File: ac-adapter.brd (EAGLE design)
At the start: 113 x 52.7 mm, 96 parts, among them IC1 UCC256404A, IC2 TL431, Q1 200V 3A, Q3 TLP621-1, T1 COMMON_FILTER-SU10VFC, T2 TRANSFORMAER_FLYBACK-ETD34

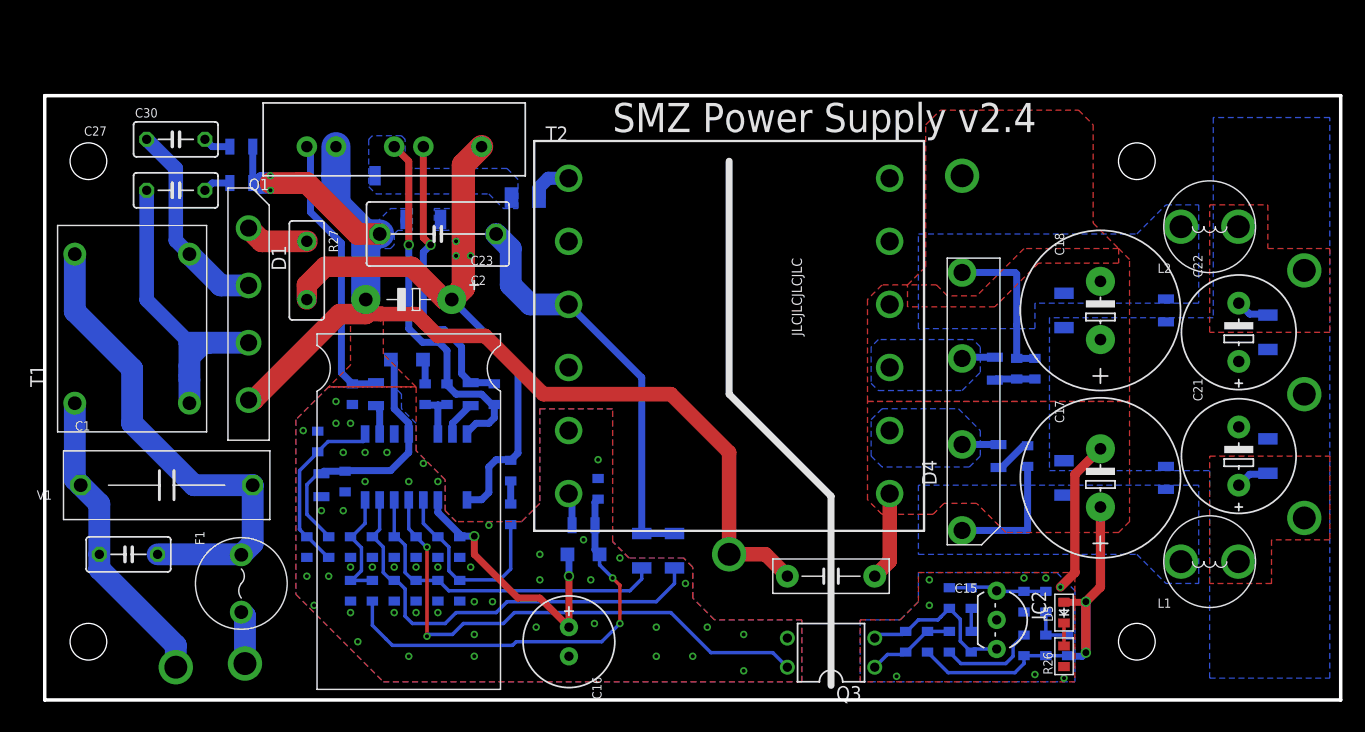
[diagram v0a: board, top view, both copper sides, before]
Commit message: 曲げた
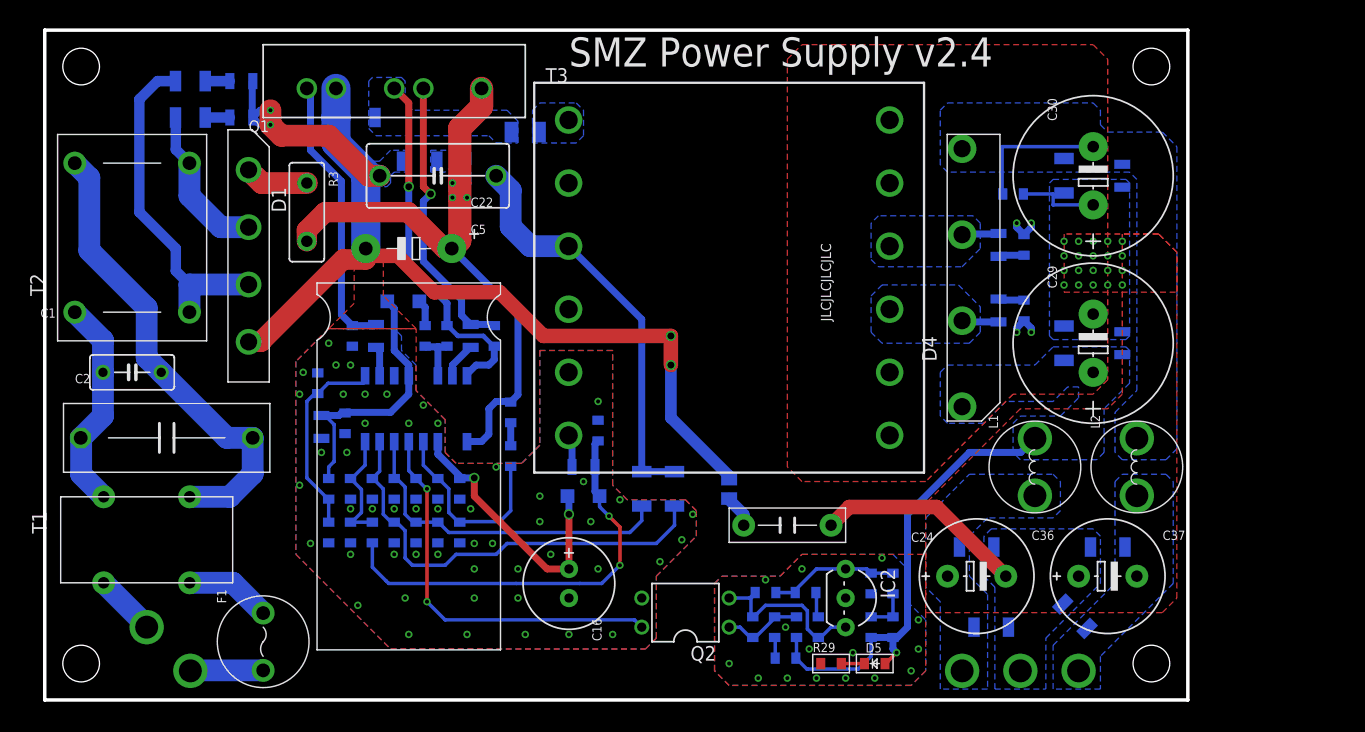
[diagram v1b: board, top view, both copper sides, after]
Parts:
- removed Q3: TLP621-1, my_ic:DIL04
- removed TP6: GND, my_connector:TESTPIN-LARGE
- removed TP7: PGND, my_connector:TESTPIN-LARGE
- removed V1: Varistor, my_rcl:C050
- added C40, C41, C42: 10u, my_rcl:3225-2
- added FB2: FB-3216, my_rcl:3216-J
- added Q2: TLP621-1, my_ic:DIL04
- added T3: TRANSFORMAER_FLYBACK-ETD34, my_rcl:BETD34LLC
- C1: value 0.22uX -> Varistor; device my_rcl:X-CAPACITER -> my_rcl:C050
- C10: value 10p -> 1u
- C11: value DNP -> 0.1u
- C12: value 22p -> 10u; device my_rcl:1608 -> my_rcl:2012
- C13: value 1kV 1000p -> 1u; device my_rcl:3225 -> my_rcl:1608
- C14: value 10p -> 1kV 1000p; device my_rcl:1608 -> my_rcl:3225
- C15: value 1000pY -> 1kV 1000p; device my_rcl:Y-CAPACITER -> my_rcl:3225
- C17: value 1000u -> 220p 1kV; device my_rcl:E5-13 -> my_rcl:3225
- C18: value 1000u -> 10p; device my_rcl:E5-13 -> my_rcl:1608
- C19: value 1000p -> 100p 1kV; device my_rcl:1608 -> my_rcl:3225
- C2: value 200V100uF -> 0.22uX; device my_rcl:E5-16A3 -> my_rcl:X-CAPACITER
- C20: value 1000p -> 6.8n
- C21: value 470u -> DNP; device my_rcl:E5-10 -> my_rcl:1608
- C22: value 470u -> 450V 0.047uF; device my_rcl:E5-10 -> my_rcl:C125
- C23: value 400V 0.01uF -> 1000p; device my_rcl:C125 -> my_rcl:1608
- C24: value 10n -> 1000pY; device my_rcl:1608 -> my_rcl:Y-CAPACITER
- C25: value 1u -> 470p
- C26: value DNP -> 470p
- C27: value 1000pX -> 1u; device my_rcl:C050 -> my_rcl:2012-2
- C28: value DNP -> 1u; device my_rcl:1608 -> my_rcl:2012-2
- C29: value 1kV 1000p -> 1000u; device my_rcl:3225 -> my_rcl:E5-13
- C3, C4: value 0.1u -> 1000pX; device my_rcl:1608 -> my_rcl:3216
- C30: value 1000pX -> 1000u; device my_rcl:C050 -> my_rcl:E5-13
- C31: value 470p -> DNP
- C32: value 10u -> DNP; device my_rcl:2012 -> my_rcl:1608
- C35: value 10u -> 10n; device my_rcl:3225-2 -> my_rcl:1608
- C36: value 10u -> 470u; device my_rcl:3225-2 -> my_rcl:E5-10
- C37: value 1u -> 470u; device my_rcl:2012-2 -> my_rcl:E5-10
- C38: value 1u -> DNP; device my_rcl:2012-2 -> my_rcl:1608
- C39: value DNP -> 10u; device my_rcl:1608 -> my_rcl:3225-2
- C5: value 1u -> 200V220uF; device my_rcl:1608 -> my_rcl:E5-16A3
- C6: value 220p 1kV -> 470p; device my_rcl:3225 -> my_rcl:1608
- C7: value 100p 1kV -> 10p; device my_rcl:3225 -> my_rcl:1608
- C8: value 6.8n -> 22p
- C9: value 1000p -> 0.1u
- D2: value 100V0.1A -> 600V1A
- D3: value 600V1A -> 100V0.1A
- FB1: value FB-1608FB -> FB2012-FB; device my_rcl:1608-FB -> my_rcl:2012-FB
- FB3: value FB-3216 -> FB2012-FB; device my_rcl:3216-J -> my_rcl:2012-FB
- R1, R2: value 120 -> 10
- R10: value 10 -> 120
- R11: value 15k -> 120; device my_rcl:1608 -> my_rcl:2012
- R12: value DNP -> 10k
- R13, R29: value 10 -> 10k; device my_rcl:2012 -> my_rcl:1608
- R14: value 1.5k -> 120
- R15: value 1.5k -> DNP
- R16: value 10k -> 22k
- R17: value 1.5k -> 3.3k
- R18: value 1.5k -> 10; device my_rcl:1608 -> my_rcl:2012
- R19, R20: value 10k -> 10; device my_rcl:1608 -> my_rcl:2012
- R22: value 3.3k -> 1.5k
- R23: value 120 -> 1.5k
- R24: value 10k -> DNP
- R25: value 240k -> 10k
- R27: value Thermistor -> 1.5k; device my_rcl:THERMISTOR090 -> my_rcl:1608
- R28: value 10 -> 1.5k; device my_rcl:2012 -> my_rcl:1608
- R3: value 39 -> Thermistor; device my_rcl:1608 -> my_rcl:THERMISTOR090
- R4: value 10 -> 240k; device my_rcl:2012 -> my_rcl:1608
- R9: value DNP -> 39
- T1: value COMMON_FILTER-SU10VFC -> COMMON_FILTER-SMALL; device my_rcl:SU10VFC -> my_rcl:COMMON_FILTER__SMALL
- T2: value TRANSFORMAER_FLYBACK-ETD34 -> COMMON_FILTER-SU10VFC; device my_rcl:BETD34LLC -> my_rcl:SU10VFC
- moved DR2 92.7 mm to (96.5, 3.17)
- moved DR3 92.1 mm to (3.17, 3.17)
- moved C27 83.6 mm to (94.0, 31.1), flipped to the bottom, turned to 90 degrees
- moved C30 80.1 mm to (91.4, 45.7), turned to 90 degrees
- moved C21 74.0 mm to (30.5, 14.6), flipped to the bottom, turned to 270 degrees
- moved C22 71.2 mm to (34.3, 45.7), turned to 180 degrees
- moved R29 68.4 mm to (68.6, 3.17), flipped to the top
- moved C18 67.2 mm to (26.7, 18.4), flipped to the bottom, turned to 270 degrees
- moved R28 65.1 mm to (72.1, 10.2), turned to 90 degrees
- moved R21 60.2 mm to (84.5, 44.1), turned to 0 degrees
- moved C26 60.1 mm to (85.4, 34.0)
- moved R16 59.6 mm to (28.6, 14.6)
- moved C29 59.4 mm to (91.4, 31.1), flipped to the top, turned to 90 degrees
- moved R27 58.0 mm to (74.0, 10.2), flipped to the bottom
- moved C15 57.5 mm to (27.3, 50.8), flipped to the bottom, turned to 0 degrees
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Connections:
- removed net N$40: C11.2, C17.+, C19.2, C33.1, C37.1, C39.2, D4.1, D5.A, L1.2, R16.2, R17.1
- removed net N$7: C18.-, C20.2, C34.2, C38.2, D4.4, L2.2, R24.1
- new net N$19: C1.1, C2.1, T1.3, T2.1
- new net N$28: C1.2, C2.2, T1.2, T2.4
- new net N$31: C24.2, FB3.2
- new net V+FIL: C36.+, C39.1, C41.1, L1.1, TP3.1
- new net V-FIL: C37.-, C40.2, C42.2, L2.1, TP4.1
- net GND: now also C24.1, C25.2, C26.2, C27.2, C28.1, C29.-, C30.+, C36.-, C37.+, C39.2, C40.1, C41.2, C42.1, R21.1, R28.1, R29.1, T3.11, T3.8; no longer C15.1, C17.-, C18.+, C21.-, C22.+, C35.2, C36.1, C37.2, C38.1, R14.1, R26.1, T2.10, T2.7, TP6.1
- net N$1: now also T1.4; no longer C1.1, T1.1, V1.1
- net N$10: now also C25.1, R19.2; no longer C20.1, R10.2, R24.2
- net N$11: now also C3.2, R1.2; no longer C27.2, R28.2
- net N$12: now also R11.2; no longer R2.2
- net N$13: now also C14.1; no longer C29.1
- net N$14: now also C11.1, R9.1; no longer C3.1, R3.1
- net N$15: now also D2.2, R9.2; no longer D3.2, R3.2
- net N$16: now also C12.1, C9.1, D2.1; no longer C32.1, C4.1, D3.1
- net N$17: now also C10.1; no longer C5.1
- net N$18: now also C6.1, R5.1; no longer C31.1, R25.1
- net N$2: now also R10.2, R12.1; no longer R1.2, R20.1
- net N$20: now also R10.1; no longer R1.1
- net N$21: now also R4.1, R5.2; no longer R25.2, R5.1
- net N$22: now also R18.2, T3.6; no longer R4.2, T2.6
- net N$23: now also C31.1, R24.2; no longer C11.1, R12.2
- net N$24: now also C23.1, D3.1, R16.2, R18.1; no longer C9.1, D2.1, R11.2, R4.1
- net N$25: now also R3.1; no longer R27.1
- net N$26: now also T1.1; no longer C1.2, T1.4, V1.2
- net N$27: now also FB2.2, T3.1; no longer FB3.2, T2.1
- net N$29: now also C32.2, Q2.2, R22.1, R25.1; no longer C28.2, Q3.2, R18.1, R19.1
- net N$3: now also C26.1, R20.1; no longer C19.1, R13.1
- net N$32: now also C32.1, C35.2, R27.1, R28.2; no longer C24.2, C28.1, R14.2, R15.1
- net N$33: now also C35.1, R25.2; no longer C24.1, R19.2
- net N$34: now also Q2.1, R22.2, R23.2, R24.1; no longer Q3.1, R12.1, R17.2, R18.2
- net N$35: now also R20.2, T3.9; no longer R13.2, T2.8
- net N$36: now also R19.1, T3.10; no longer R10.1, T2.9
- net N$37: now also R29.2; no longer R26.2
- net N$38: now also C4.2, R2.2; no longer C30.2, R29.2
- net N$4: now also C3.1, T2.2; no longer C27.1, T1.2
- net N$5: now also C4.1, T2.3; no longer C30.1, T1.3
- net N$6: now also C38.1, R26.1, R27.2; no longer C39.1, R15.2, R16.1
- net N$8: now also C17.1, C19.1, C22.1, T3.3; no longer C23.1, C6.1, C7.1, T2.3
- net N$9: now also R11.1, R13.2; no longer R2.1, R21.2
- net PGND: now also C18.2, C20.2, C21.2, C22.2, C5.-, C6.2, C7.2, FB3.1, Q2.3, R1.1, R13.1, R14.1, R15.1, R17.1, R2.1, T3.5; no longer C2.-, C25.2, C26.2, C29.2, C31.2, C32.2, C4.2, C5.2, Q3.3, R21.1, R22.1, R23.1, R28.1, R29.1, R9.1, T2.5, TP7.1
- net SW: now also C11.2, C15.1, FB2.1, R12.2; no longer C13.1, C3.2, FB3.1, R20.2
- net UCC_BW: now also C18.1, R16.1, R17.2; no longer C14.1, R11.1, R22.2
- net UCC_FB: now also C8.1, Q2.4; no longer C12.1, Q3.4
- net UCC_ISNS: now also C17.2, C7.1, R14.2, R15.2; no longer C10.1, C6.2, R23.2, R9.2
- net UCC_VCC: now also C13.1, D3.2; no longer C25.1, D2.2
- net UCC_VCR: now also C19.2, C20.1, C21.1; no longer C26.1, C7.2, C8.1
- net V+: now also C27.1, C29.+, C31.2, C33.1, C38.2, D4.1, D5.A, L1.2, R23.1, R26.2; no longer C21.+, C35.1, L1.1, TP3.1
- net V-: now also C28.2, C30.-, C34.2, D4.4, L2.2, R21.2; no longer C22.-, C36.2, L2.1, TP4.1
- net VH: now also C5.+, R3.2, R4.2; no longer C2.+, R27.2, R5.2
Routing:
- net N$40: track 46.7 -> 0.00 mm, vias 2 -> 0
- net N$28: track 0.00 -> 41.2 mm
- net V+: track 2.97 -> 41.0 mm, vias 0 -> 1
- net N$26: track 43.4 -> 7.50 mm
- net N$1: track 26.7 -> 5.42 mm
- net N$19: track 0.00 -> 18.8 mm
- net N$7: track 13.8 -> 0.00 mm
- net UCC_FB: track 46.8 -> 34.3 mm
- net GND: track 21.3 -> 30.5 mm, vias 8 -> 39
- net V-: track 2.97 -> 12.1 mm
- net N$23: track 8.48 -> 1.82 mm
- net PGND: track 101.8 -> 97.1 mm, vias 50 -> 55
- net N$5: track 17.8 -> 13.7 mm
- net N$27: track 3.79 -> 0.00 mm
- net N$31: track 0.00 -> 2.85 mm
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- added copper zone on layer 16, net N$27
- added copper zone on layer 16, net V+
- added copper zone on layer 16, net V+FIL
- added copper zone on layer 16, net V-
- added copper zone on layer 16, net V-FIL
- removed copper zone on layer 16, net N$40
- removed copper zone on layer 16, net N$7
- removed copper zone on layer 1, net V+
- removed copper zone on layer 1, net V-
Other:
- board size 113 x 52.7 mm -> 99.7 x 58.4 mm
